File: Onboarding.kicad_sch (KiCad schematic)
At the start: 0 parts

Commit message: Test Commit
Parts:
- added C1: 100u, symbol Device:C
- added R1: 180, symbol Device:R
- added RSC: .22, symbol Device:R
- added U2: MC34063A, Package_SO:SOIC-8_3.9x4.9mm_P1.27mm, symbol ! Robomaster ICs:MC34063A

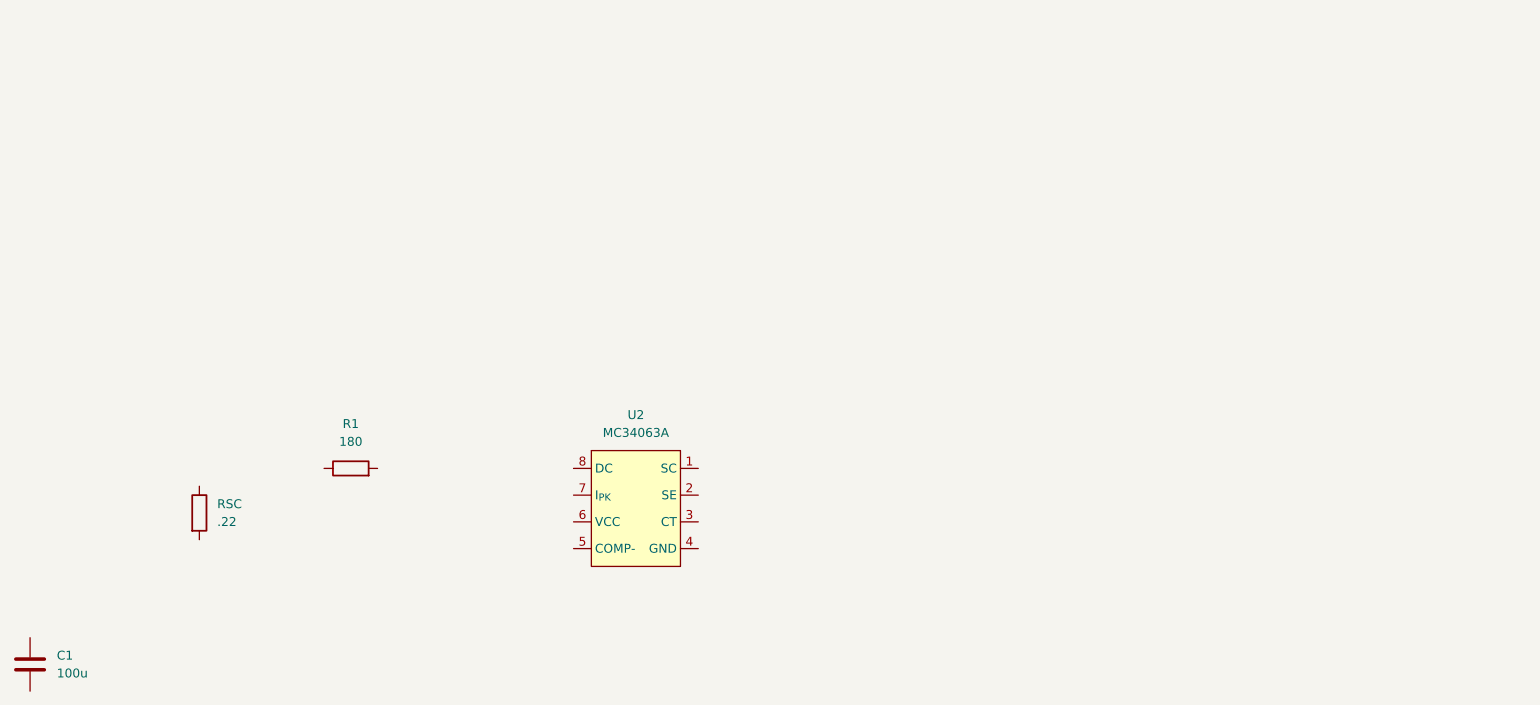
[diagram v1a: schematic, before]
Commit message: Update Onboarding.kicad_sch
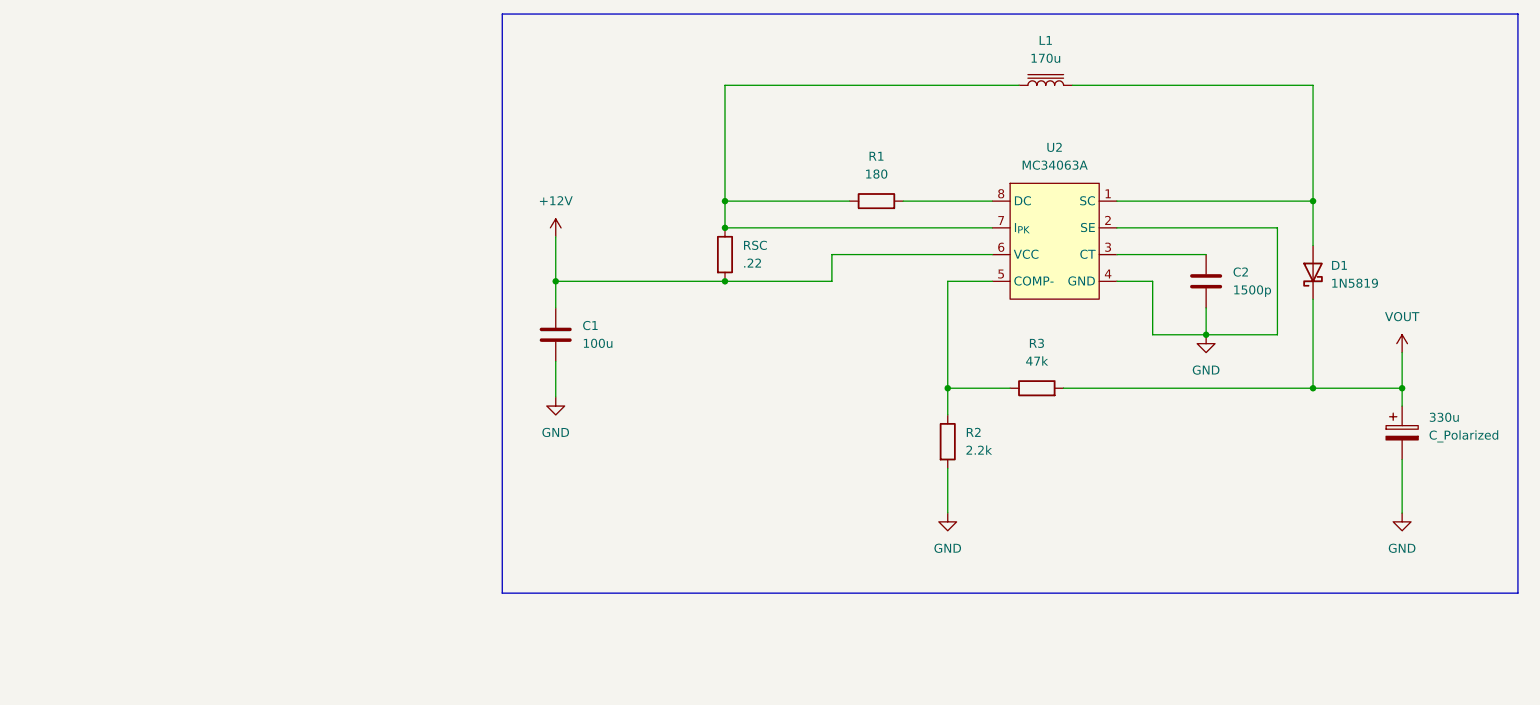
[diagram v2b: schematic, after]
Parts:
- added 330u: C_Polarized, symbol Device:C_Polarized
- added C2: 1500p, symbol Device:C
- added D1: 1N5819, Diode_THT:D_DO-41_SOD81_P10.16mm_Horizontal, symbol Diode:1N5819
- added L1: 170u, symbol Device:L_Iron
- added R2: 2.2k, symbol Device:R
- added R3: 47k, symbol Device:R
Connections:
- net at U2.1 (SC): now also D1.2 (A), L1.2
- net GND: now reaches U2.2 (SE)
- net GND: now also C1.2, U2.4 (GND), 330u.2, C2.2, R2.2
- net at U2.3 (CT): now also C2.1
- net at U2.5 (COMP-): now also R2.1, R3.1
- net +12V: now reaches U2.6 (VCC)
- net +12V: now also C1.1, RSC.2
- net at U2.7 (I_{PK}): now also R1.1, RSC.1, L1.1
- net at U2.8 (DC): now also R1.2
- new net VOUT: 330u.1, D1.1 (K), R3.2
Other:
- moved on the sheet: C1, R1, RSC, U2
